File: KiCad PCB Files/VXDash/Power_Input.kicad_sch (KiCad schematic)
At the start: 20 parts, among them Q5 2N7002, Q6 PJA3441, Q7 PJA3441

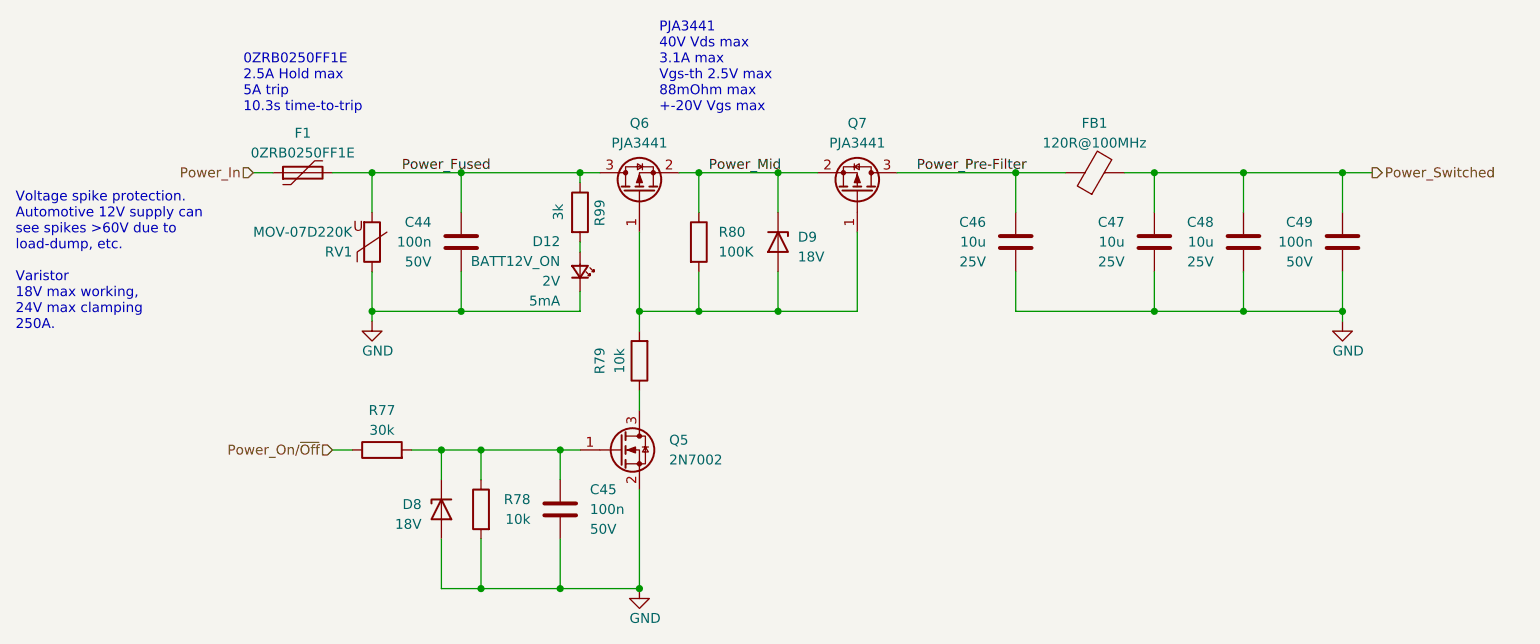
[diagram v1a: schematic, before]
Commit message: BOM first pass
- Still missing some internal connectors definitions
- Alternative to use a 4x4ch opto config instead of 16x1 ?
- Alternative LiteOn optos identified (easier to source on LCSC)
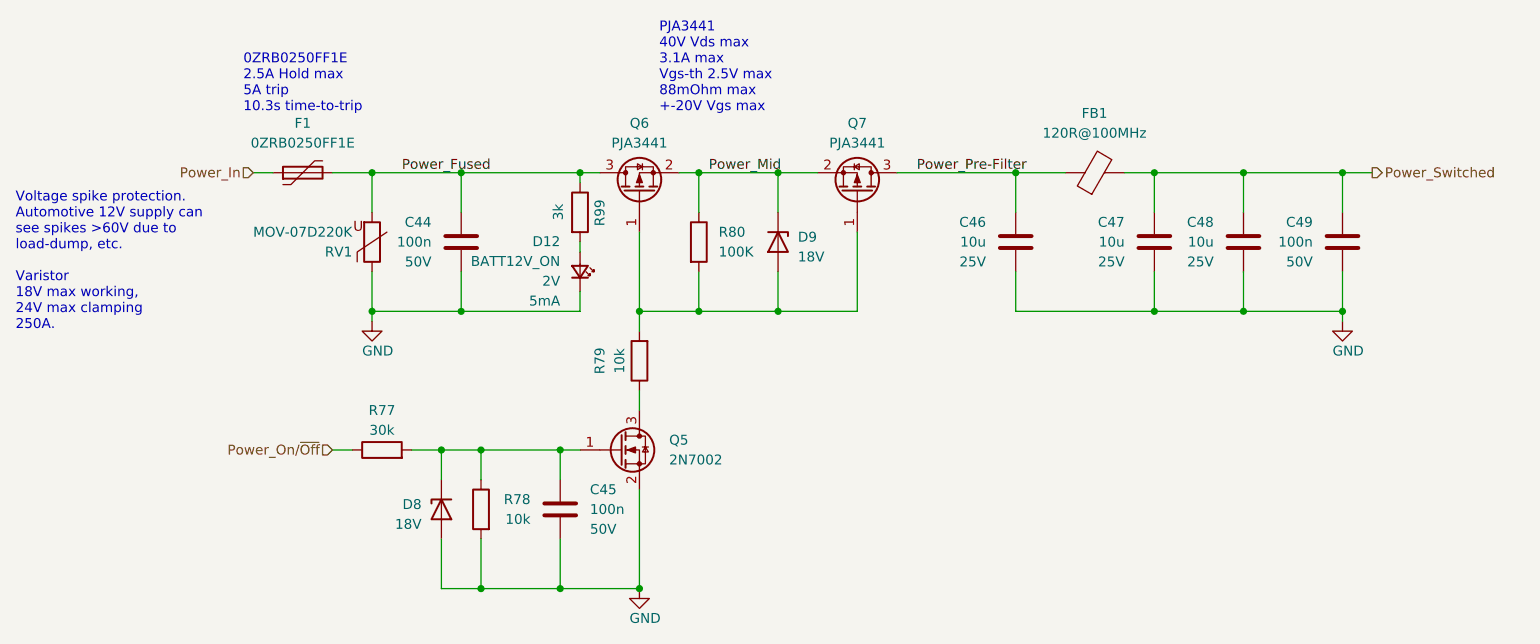
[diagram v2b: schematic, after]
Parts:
- C44, C45, C49: LCSC (none) -> C16194176; MFT (none) -> Samsung Electro-Mechanics; MFT_PN (none) -> CL10B104KB8NNWC
- C46, C47, C48: LCSC (none) -> C14860; MFT (none) -> Samsung Electro-Mechanics; MFT_PN (none) -> CL31B106KAHNNNE
- D12: LCSC (none) -> C157740; MFT (none) -> Lite-On; MFT_PN (none) -> LTST-C190KFKT
- D8, D9: ALT_MFT_PN_1 (none) -> BZT52C18-E3-08; LCSC (none) -> C668896; LCSC alt (none) -> C467525
- F1: LCSC (none) -> C3761262; LCSC alt (none) -> C207101
- FB1: ALT_MFT_PN_1 (none) -> BLM21PG121SN1D; LCSC (none) -> N/A; LCSC alt (none) -> C79382
- Q5: LCSC (none) -> C78712
- Q6, Q7: LCSC (none) -> C313504
- R77: LCSC (none) -> C126352; MFT (none) -> Yageo; MFT_PN (none) -> RC0805FR-0730KL; Power 100mW -> 125mW
- R78, R79: LCSC (none) -> C98220; MFT (none) -> Yageo; MFT_PN (none) -> RC0603FR-0710KL
- R80: LCSC (none) -> C14675; MFT (none) -> Yageo; MFT_PN (none) -> RC0603FR-07100KL
- R99: LCSC (none) -> C126358; MFT (none) -> Yageo; MFT_PN (none) -> RC0603FR-073KL
- RV1: LCSC (none) -> C1528486
